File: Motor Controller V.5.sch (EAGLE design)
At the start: 54 parts, among them IC1 MEGA8-P, J1 NMJ6HCD2-RM, Q1 IRF540

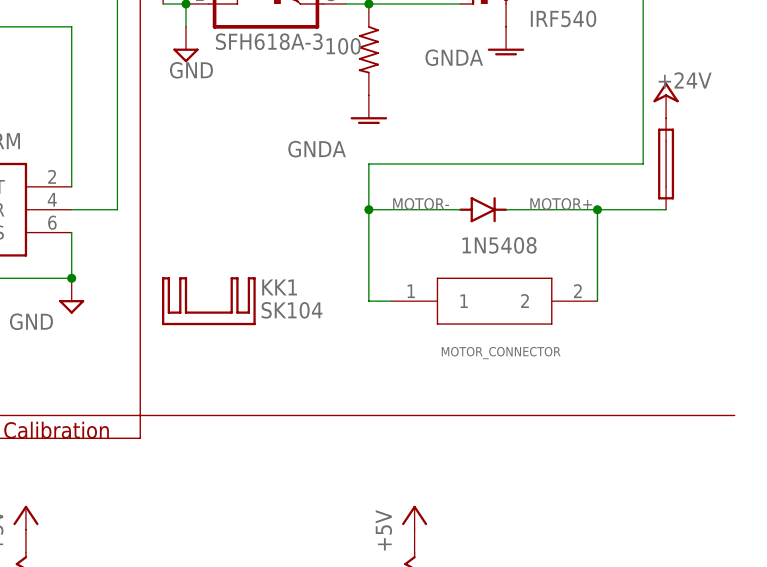
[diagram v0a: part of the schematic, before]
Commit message: Starting to route on new board with updated components. v5.1
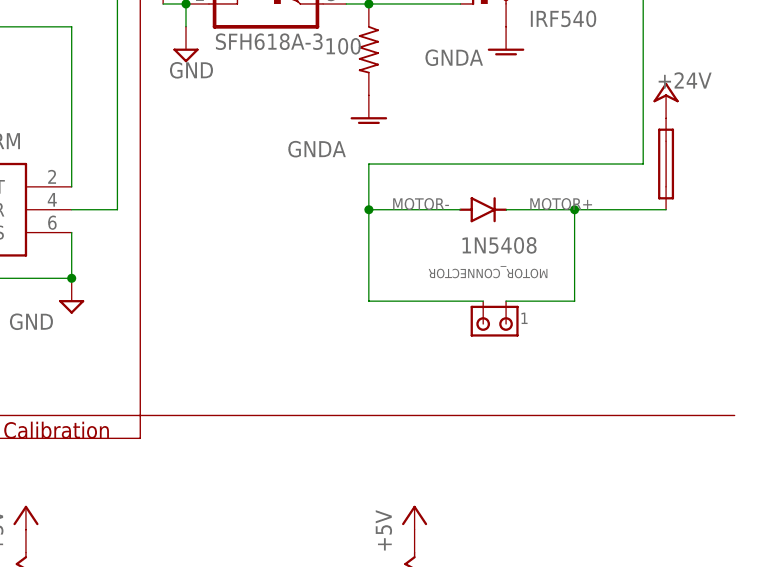
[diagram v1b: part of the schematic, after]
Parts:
- removed KK1: SK104, Benson Motor Controller:SK104
- MOTOR_CONNECTOR: value 641963-1 -> MATE-N-LOK_193839-1; device Benson:641963-1 -> Benson Motor Controller:MATE-N-LOK_193839-1
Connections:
- net MOTOR+: now also MOTOR_CONNECTOR.1; no longer MOTOR_CONNECTOR.2
- net MOTOR-: now also MOTOR_CONNECTOR.2; no longer MOTOR_CONNECTOR.1
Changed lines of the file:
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@@
 </part>
 <part name="GND2" library="supply1" library_urn="urn:adsk.eagle:library:371" deviceset="GNDA" device=""/>
-<part name="MOTOR_CONNECTOR" library="Benson" deviceset="641963-1" device="">
+<part name="MOTOR_CONNECTOR" library="Benson Motor Controller" deviceset="MATE-N-LOK_193839-1" device="">
 <attribute name="MF" value=""/>
 <attribute name="MPN" value=""/>
@@
 <part name="P+4" library="supply1" library_urn="urn:adsk.eagle:library:371" deviceset="+24V" device=""/>
 <part name="P+10" library="supply1" library_urn="urn:adsk.eagle:library:371" deviceset="+24V" device=""/>
-<part name="KK1" library="Benson Motor Controller" deviceset="SK104" device="" package3d_urn="urn:adsk.eagle:package:14176/1">
-<attribute name="MF" value=""/>
-<attribute name="MPN" value=""/>
-<attribute name="OC_NEWARK" value="unknown"/>
-</part>
 <part name="PS1" library="Benson Motor Controller" deviceset="PBO-15C-24" device="">
 <attribute name="MPN" value=""/>
@@
 <attribute name="VALUE" x="149.86" y="104.14" size="1.778" layer="96" rot="R180"/>
 </instance>
-<instance part="MOTOR_CONNECTOR" gate="A" x="149.86" y="76.2" smashed="yes">
-<attribute name="NAME" x="145.1356" y="70.0786" size="1.016" layer="95" ratio="6" rot="SR0"/>
-<attribute name="OC_NEWARK" x="149.86" y="76.2" size="1.778" layer="96" display="off"/>
-<attribute name="MF" x="149.86" y="76.2" size="1.778" layer="96" display="off"/>
-<attribute name="MPN" x="149.86" y="76.2" size="1.778" layer="96" display="off"/>
+<instance part="MOTOR_CONNECTOR" gate="G$1" x="152.4" y="73.66" smashed="yes" rot="R180">
+<attribute name="NAME" x="157.1244" y="79.7814" size="1.016" layer="95" ratio="6" rot="SR180"/>
+<attribute name="OC_NEWARK" x="152.4" y="73.66" size="1.778" layer="96" rot="R180" display="off"/>
+<attribute name="MF" x="152.4" y="73.66" size="1.778" layer="96" rot="R180" display="off"/>
+<attribute name="MPN" x="152.4" y="73.66" size="1.778" layer="96" rot="R180" display="off"/>
 </instance>
 <instance part="1N5408" gate="1" x="149.86" y="86.36" smashed="yes">
@@
 <instance part="P+10" gate="1" x="170.18" y="99.06" smashed="yes">
 <attribute name="VALUE" x="175.26" y="101.6" size="1.778" layer="96" rot="R180"/>
-</instance>
-<instance part="KK1" gate="1" x="119.38" y="73.66" smashed="yes">
-<attribute name="NAME" x="125.095" y="76.835" size="1.778" layer="95"/>
-<attribute name="VALUE" x="125.095" y="74.295" size="1.778" layer="96"/>
-<attribute name="OC_NEWARK" x="119.38" y="73.66" size="1.778" layer="96" display="off"/>
-<attribute name="MF" x="119.38" y="73.66" size="1.778" layer="96" display="off"/>
-<attribute name="MPN" x="119.38" y="73.66" size="1.778" layer="96" display="off"/>
 </instance>
 <instance part="PS1" gate="G$1" x="35.56" y="30.48" smashed="yes">
@@
 <wire x1="152.4" y1="119.38" x2="167.64" y2="119.38" width="0.1524" layer="91"/>
 <wire x1="167.64" y1="119.38" x2="167.64" y2="91.44" width="0.1524" layer="91"/>
-<pinref part="MOTOR_CONNECTOR" gate="A" pin="1"/>
 <wire x1="137.16" y1="91.44" x2="137.16" y2="86.36" width="0.1524" layer="91"/>
 <wire x1="137.16" y1="86.36" x2="137.16" y2="76.2" width="0.1524" layer="91"/>
-<wire x1="137.16" y1="76.2" x2="139.7" y2="76.2" width="0.1524" layer="91"/>
 <label x="139.7" y="86.36" size="1.27" layer="95" ratio="6"/>
 <wire x1="167.64" y1="91.44" x2="137.16" y2="91.44" width="0.1524" layer="91"/>
@@
 <wire x1="147.32" y1="86.36" x2="137.16" y2="86.36" width="0.1524" layer="91"/>
 <junction x="137.16" y="86.36"/>
+<pinref part="MOTOR_CONNECTOR" gate="G$1" pin="2"/>
+<wire x1="137.16" y1="76.2" x2="149.86" y2="76.2" width="0.1524" layer="91"/>
 </segment>
 </net>
@@
 <segment>
 <pinref part="1N5408" gate="1" pin="C"/>
-<wire x1="152.4" y1="86.36" x2="162.56" y2="86.36" width="0.1524" layer="91"/>
+<wire x1="152.4" y1="86.36" x2="160.02" y2="86.36" width="0.1524" layer="91"/>
 <pinref part="F1" gate="G$1" pin="1"/>
 <label x="154.94" y="86.36" size="1.27" layer="95" ratio="6"/>
-<pinref part="MOTOR_CONNECTOR" gate="A" pin="2"/>
-<wire x1="162.56" y1="86.36" x2="170.18" y2="86.36" width="0.1524" layer="91"/>
-<wire x1="162.56" y1="76.2" x2="162.56" y2="86.36" width="0.1524" layer="91"/>
-<junction x="162.56" y="86.36"/>
-</segment>
-</net>
+<pinref part="MOTOR_CONNECTOR" gate="G$1" pin="1"/>
+<wire x1="160.02" y1="86.36" x2="170.18" y2="86.36" width="0.1524" layer="91"/>
+<wire x1="152.4" y1="76.2" x2="160.02" y2="76.2" width="0.1524" layer="91"/>
+<wire x1="160.02" y1="76.2" x2="160.02" y2="86.36" width="0.1524" layer="91"/>
+<junction x="160.02" y="86.36"/>
+</segment>
+</net>
